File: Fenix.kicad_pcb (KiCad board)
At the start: 2 copper layers, 73.5 x 54 mm, 5 parts

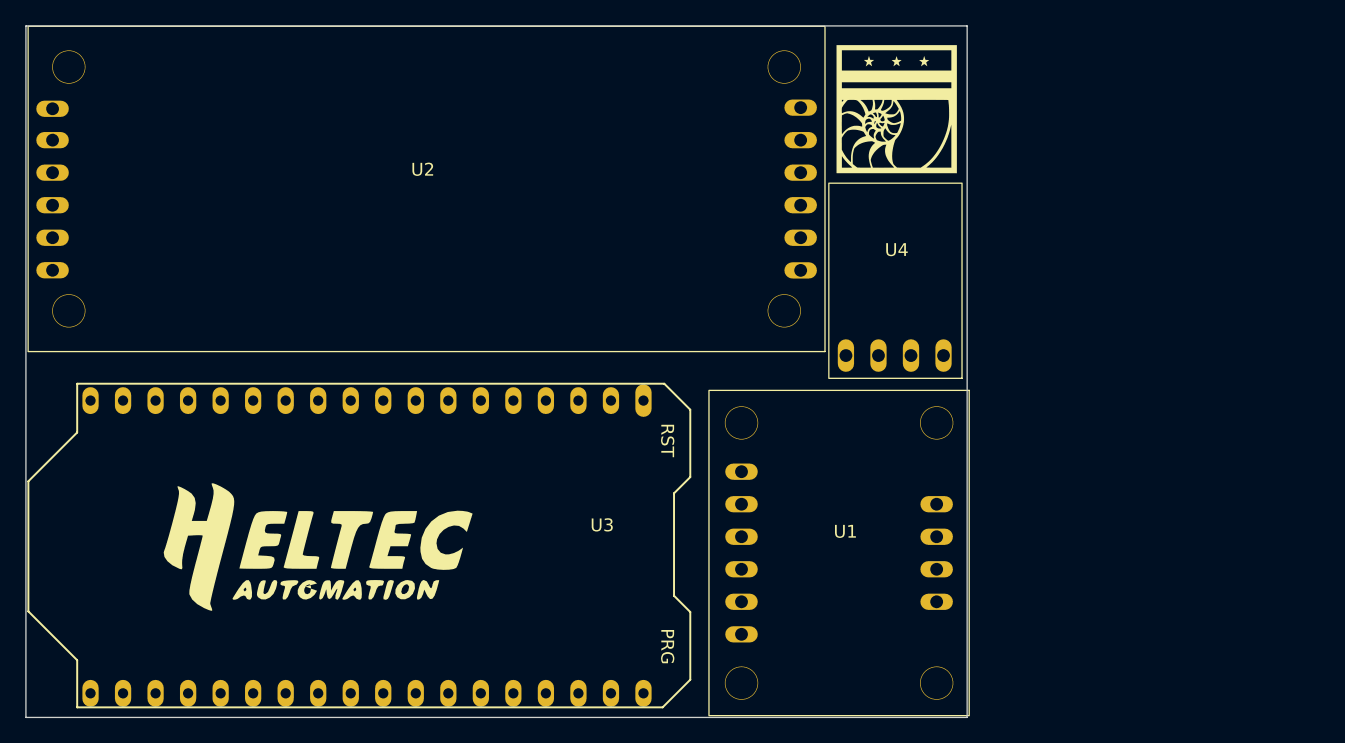
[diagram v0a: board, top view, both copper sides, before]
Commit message: Completed parts library
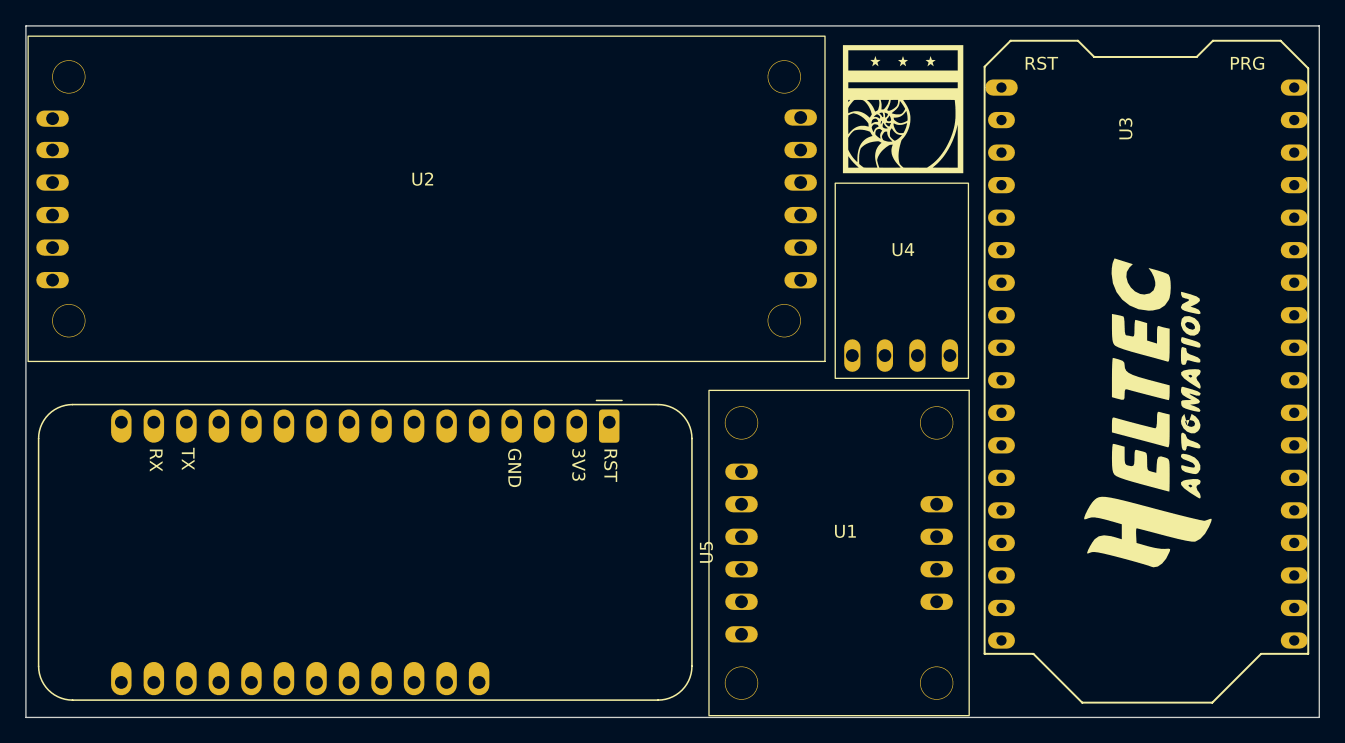
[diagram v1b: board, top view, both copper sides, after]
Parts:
- added U5: ~, Parts:Adafruit_GPSFeather, F.Cu at (119.5, 84.9)
- moved U3 60.7 mm to (161.4, 78.0), turned to 0 degrees
- moved U2 0.77 mm to (105.3, 67.5)
- moved G*** 0.50 mm to (142.5, 60.5)
- moved U4 0.50 mm to (147.6, 81.5)
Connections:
- U1 pad 1: (no net) -> unconnected-(U1-VIN-Pad1)
- U1 pad 10: (no net) -> unconnected-(U1-PS0-Pad10)
- U1 pad 2: (no net) -> +3V3
- U1 pad 3: (no net) -> GND
- U1 pad 4: (no net) -> unconnected-(U1-SDA-Pad4)
- U1 pad 5: (no net) -> unconnected-(U1-SCL-Pad5)
- U1 pad 6: (no net) -> unconnected-(U1-RST-Pad6)
- U1 pad 7: (no net) -> unconnected-(U1-ADR-Pad7)
- U1 pad 8: (no net) -> unconnected-(U1-INT-Pad8)
- U1 pad 9: (no net) -> unconnected-(U1-PS1-Pad9)
- U2 pad 1: (no net) -> GND
- U2 pad 10: (no net) -> unconnected-(U2-SCL-Pad10)
- U2 pad 11: (no net) -> unconnected-(U2-OE-Pad11)
- U2 pad 12: (no net) -> GND
- U2 pad 2: (no net) -> unconnected-(U2-OE-Pad2)
- U2 pad 3: (no net) -> unconnected-(U2-SCL-Pad3)
- U2 pad 4: (no net) -> unconnected-(U2-SDA-Pad4)
- U2 pad 5: (no net) -> +3V3
- U2 pad 6: (no net) -> +5V
- U2 pad 7: (no net) -> +5V
- U2 pad 8: (no net) -> +3V3
- U2 pad 9: (no net) -> unconnected-(U2-SDA-Pad9)
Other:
- board size 73.5 x 54 mm -> 101 x 54 mm
